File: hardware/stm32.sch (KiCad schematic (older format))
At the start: 13 parts, among them J6 PROG, U7 STM32F103C8Tx, Y1 16MHz

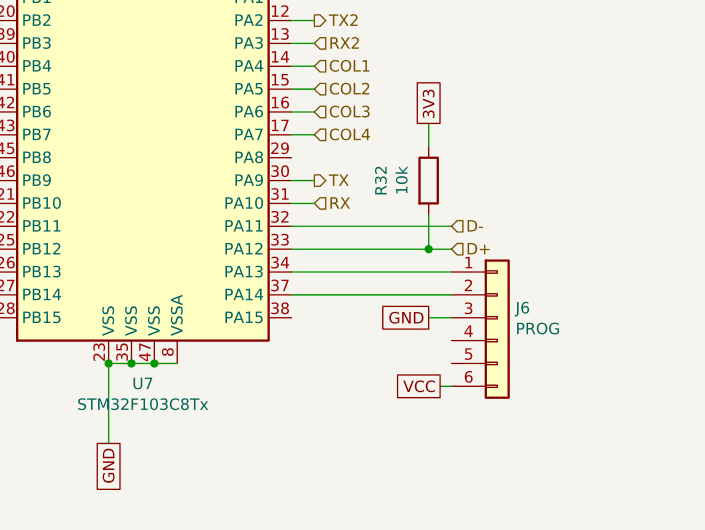
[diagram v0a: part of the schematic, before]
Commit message: Final layout changes
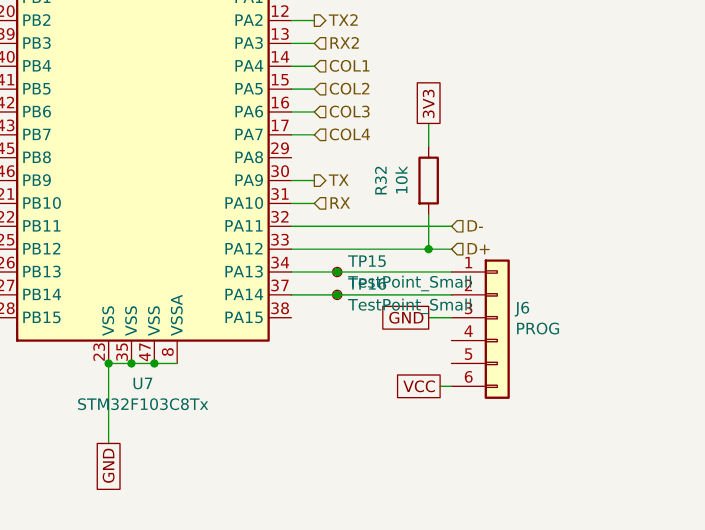
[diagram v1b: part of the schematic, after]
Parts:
- added TP15, TP16: TestPoint_Small, TestPoint:TestPoint_Pad_D1.5mm, symbol Connector:TestPoint_Small
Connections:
- net at J6.1 (Pin_1), U7.34 (PA13): now also TP15.1
- net at J6.2 (Pin_2), U7.37 (PA14): now also TP16.1
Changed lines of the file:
@@
 $EndComp
 Wire Wire Line
-	5800 4800 6500 4800
+	5800 4800 6000 4800
 Wire Wire Line
-	6500 4900 5800 4900
+	6500 4900 6000 4900
 Text GLabel 6400 5000 0    50   UnSpc ~ 0
 GND
@@
 Wire Wire Line
 	6450 5300 6500 5300
+$Comp
+L Connector:TestPoint_Small TP15
+U 1 1 5ED4800E
+P 6000 4800
+F 0 "TP15" H 6048 4846 50  0000 L CNN
+F 1 "TestPoint_Small" H 6048 4755 50  0000 L CNN
+F 2 "TestPoint:TestPoint_Pad_D1.5mm" H 6200 4800 50  0001 C CNN
+F 3 "~" H 6200 4800 50  0001 C CNN
+	1    6000 4800
+	1    0    0    -1
+$EndComp
+Connection ~ 6000 4800
+Wire Wire Line
+	6000 4800 6500 4800
+$Comp
+L Connector:TestPoint_Small TP16
+U 1 1 5ED49503
+P 6000 4900
+F 0 "TP16" H 6048 4946 50  0000 L CNN
+F 1 "TestPoint_Small" H 6048 4855 50  0000 L CNN
+F 2 "TestPoint:TestPoint_Pad_D1.5mm" H 6200 4900 50  0001 C CNN
+F 3 "~" H 6200 4900 50  0001 C CNN
+	1    6000 4900
+	1    0    0    -1
+$EndComp
+Connection ~ 6000 4900
+Wire Wire Line
+	6000 4900 5800 4900
 $EndSCHEMATC
